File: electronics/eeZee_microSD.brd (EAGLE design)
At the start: 18.3 x 19.8 mm, 13 parts, among them U1 MIC5317, U2 74HC4050, U4 MICROSD_CD

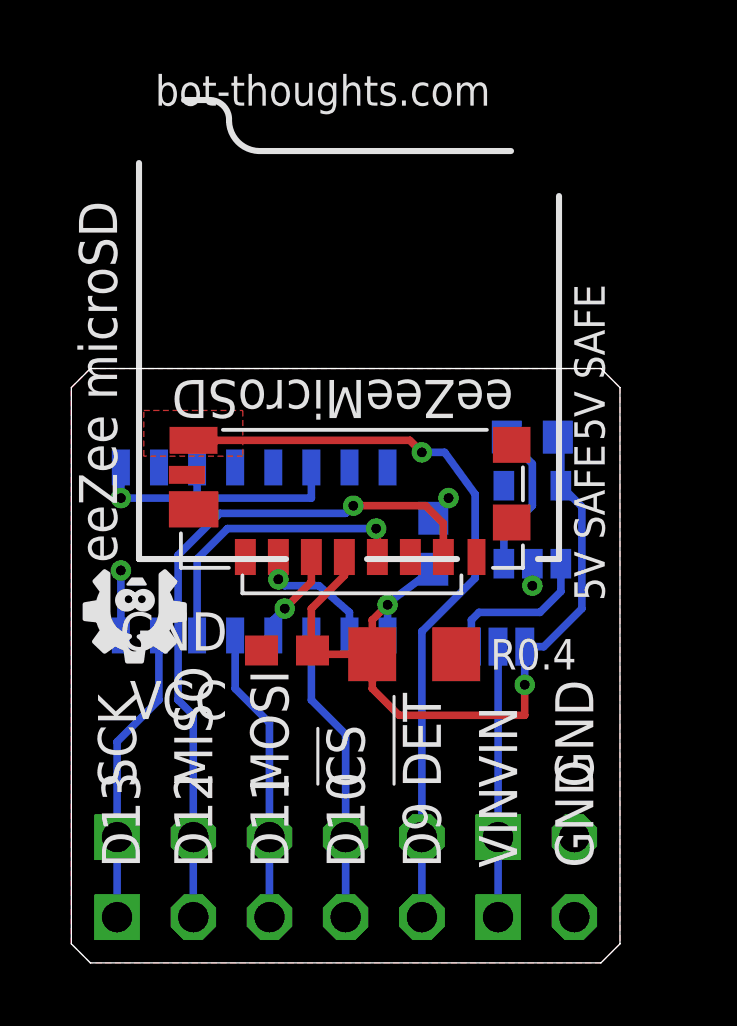
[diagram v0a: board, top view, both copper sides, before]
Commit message: rotated board
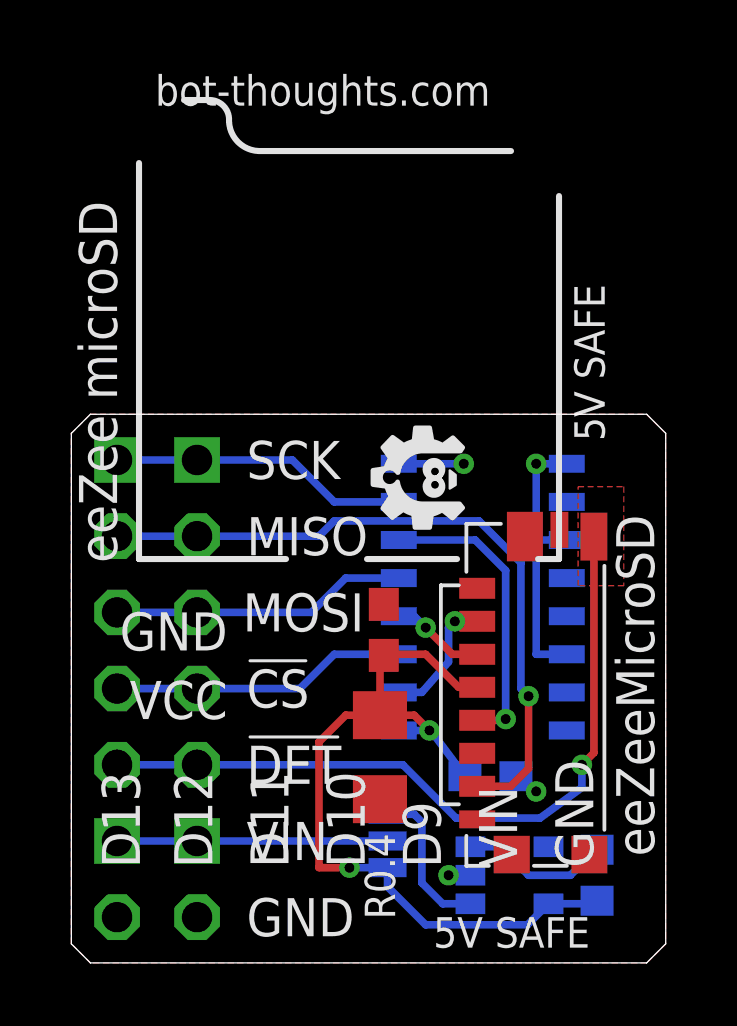
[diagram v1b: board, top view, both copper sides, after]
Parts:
- moved R5 14.8 mm to (17.5, 2.92), turned to 90 degrees
- moved JP2 14.0 mm to (1.52, 2.79), turned to 270 degrees
- moved U1 11.7 mm to (14.6, 2.92), turned to 90 degrees
- moved U$5 11.4 mm to (13.2, 16.1), turned to 90 degrees
- moved JP1 11.4 mm to (4.19, 2.79), turned to 270 degrees
- moved JP3 11.4 mm to (1.52, 11.7), turned to 270 degrees
- moved C2 7.98 mm to (14.0, 6.22), turned to 180 degrees
- moved JP4 7.87 mm to (4.19, 11.7), turned to 270 degrees
- moved U2 7.77 mm to (13.7, 12.2), turned to 90 degrees
- moved 5V 7.45 mm to (10.5, 4.06), turned to 90 degrees
- moved U4 4.55 mm to (12.3, 8.64), turned to 90 degrees
- moved C1 3.61 mm to (10.3, 6.86), turned to 270 degrees
- moved C3 3.30 mm to (10.4, 11.1), turned to 90 degrees
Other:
- board size 18.3 x 19.8 mm -> 19.8 x 18.3 mm
